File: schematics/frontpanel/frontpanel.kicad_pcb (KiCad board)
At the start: 2 copper layers, 72.4 x 21.6 mm, 10 parts, among them J1 Conn_01x02_Male, J2 Conn_01x02_Male, J3 Conn_01x03_Male, J4 Conn_01x03_Male, SW1 SW_Push, SW2 SW_Push

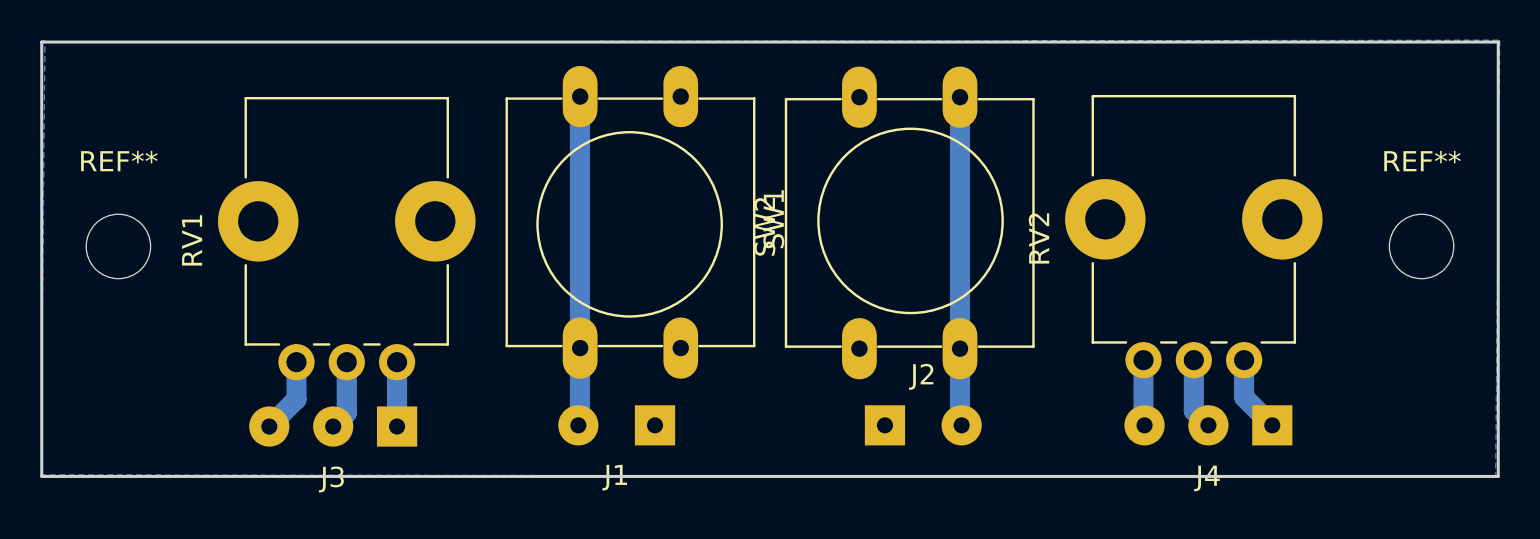
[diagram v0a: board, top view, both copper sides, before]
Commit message: PCBs updated
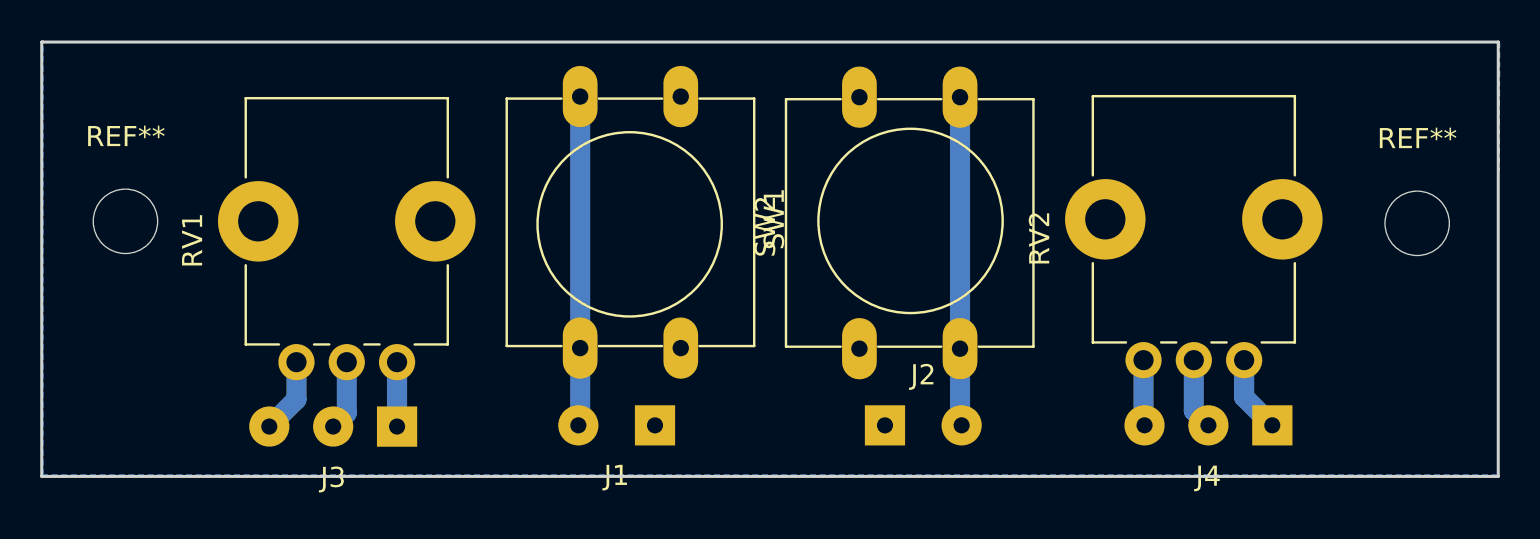
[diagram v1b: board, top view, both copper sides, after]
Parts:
- removed the REF** at (109.2, 120.7)
- removed the REF** at (44.5, 120.7)
- added REF**: MountingHole_3.2mm_M3, MountingHole:MountingHole_3.2mm_M3, F.Cu at (109.0, 119.5)
- added REF**: MountingHole_3.2mm_M3, MountingHole:MountingHole_3.2mm_M3, F.Cu at (44.8, 119.4)
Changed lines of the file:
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@@
     (thickness 1.6)
     (drawings 6)
-    (tracks 18)
+    (tracks 19)
     (zones 0)
     (modules 10)
@@
     (last_trace_width 1)
     (trace_clearance 0.5)
-    (zone_clearance 0.508)
+    (zone_clearance 0.6)
     (zone_45_only no)
     (trace_min 0.2)
@@
     (visible_elements FFFFFF7F)
     (pcbplotparams
-      (layerselection 0x010fc_ffffffff)
+      (layerselection 0x00000_fffffffe)
       (usegerberextensions false)
       (usegerberattributes false)
       (usegerberadvancedattributes false)
       (creategerberjobfile false)
-      (excludeedgelayer true)
+      (excludeedgelayer false)
       (linewidth 0.100000)
       (plotframeref false)
@@
       (hpglpenspeed 20)
       (hpglpendiameter 15.000000)
-      (psnegative false)
+      (psnegative true)
       (psa4output false)
-      (plotreference true)
-      (plotvalue true)
+      (plotreference false)
+      (plotvalue false)
       (plotinvisibletext false)
-      (padsonsilk false)
+      (padsonsilk true)
       (subtractmaskfromsilk false)
-      (outputformat 1)
+      (outputformat 4)
       (mirror false)
-      (drillshape 1)
+      (drillshape 2)
       (scaleselection 1)
       (outputdirectory ""))
@@
   )
   (module MountingHole:MountingHole_3.2mm_M3 (layer F.Cu)
-    (at 109.22 120.65)
+    (at 109 119.5)
     (descr "Mounting Hole 3.2mm, no annular, M3")
     (tags "mounting hole 3.2mm no annular m3")
@@
   )
   (module MountingHole:MountingHole_3.2mm_M3 (layer F.Cu)
-    (at 44.45 120.65)
+    (at 44.8 119.4)
     (descr "Mounting Hole 3.2mm, no annular, M3")
     (tags "mounting hole 3.2mm no annular m3")
@@
     )
     (pad 1 np_thru_hole circle (at 0 0) (size 3.2 3.2) (drill 3.2) (layers *.Cu *.Mask))
+  )
+  (dimension 72.39 (width 0.3) (layer Dwgs.User)
+    (gr_text "72,390 mm" (at 76.835 139.26) (layer Dwgs.User)
+      (effects (font (size 1.5 1.5) (thickness 0.3)))
+    )
+    (feature1 (pts (xy 113.03 132.08) (xy 113.03 137.746421)))
+    (feature2 (pts (xy 40.64 132.08) (xy 40.64 137.746421)))
+    (crossbar (pts (xy 40.64 137.16) (xy 113.03 137.16)))
+    (arrow1a (pts (xy 113.03 137.16) (xy 111.903496 137.746421)))
+    (arrow1b (pts (xy 113.03 137.16) (xy 111.903496 136.573579)))
+    (arrow2a (pts (xy 40.64 137.16) (xy 41.766504 137.746421)))
+    (arrow2b (pts (xy 40.64 137.16) (xy 41.766504 136.573579)))
   )
   (dimension 21.59 (width 0.3) (layer Dwgs.User)
@@
     (arrow2b (pts (xy 35.56 132.08) (xy 34.973579 130.953496)))
   )
-  (dimension 72.39 (width 0.3) (layer Dwgs.User)
-    (gr_text "72,390 mm" (at 76.835 139.26) (layer Dwgs.User)
-      (effects (font (size 1.5 1.5) (thickness 0.3)))
-    )
-    (feature1 (pts (xy 113.03 132.08) (xy 113.03 137.746421)))
-    (feature2 (pts (xy 40.64 132.08) (xy 40.64 137.746421)))
-    (crossbar (pts (xy 40.64 137.16) (xy 113.03 137.16)))
-    (arrow1a (pts (xy 113.03 137.16) (xy 111.903496 137.746421)))
-    (arrow1b (pts (xy 113.03 137.16) (xy 111.903496 136.573579)))
-    (arrow2a (pts (xy 40.64 137.16) (xy 41.766504 137.746421)))
-    (arrow2b (pts (xy 40.64 137.16) (xy 41.766504 136.573579)))
-  )
   (gr_line (start 40.64 132.08) (end 40.64 110.49) (layer Edge.Cuts) (width 0.15))
   (gr_line (start 113.03 132.08) (end 40.64 132.08) (layer Edge.Cuts) (width 0.15))
@@
   (segment (start 81.08 113.03) (end 81.28 113.23) (width 1) (layer B.Cu) (net 1))
   (segment (start 67.39 129.46) (end 67.31 129.54) (width 1) (layer B.Cu) (net 2))
-  (segment (start 67.39 113.03) (end 67.39 129.46) (width 1) (layer B.Cu) (net 2))
+  (segment (start 67.4 129.45) (end 67.31 129.54) (width 1) (layer B.Cu) (net 2))
+  (segment (start 67.4 113.2) (end 67.4 129.45) (width 1) (layer B.Cu) (net 2))
   (segment (start 58.3 126.4) (end 58.3 129.6) (width 1) (layer B.Cu) (net 3))
   (segment (start 55.8 128.925) (end 55.125 129.6) (width 1) (layer B.Cu) (net 4))
@@
   (segment (start 86.28 113.23) (end 86.28 129.46) (width 1) (layer B.Cu) (net 9))
   (zone (net 1) (net_name "Net-(J1-Pad1)") (layer B.Cu) (hatch edge 0.508)
-    (connect_pads (clearance 0.508))
+    (connect_pads (clearance 0.6))
     (min_thickness 0.254)
     (fill yes (arc_segments 16) (thermal_gap 0.508) (thermal_bridge_width 0.508))
     (polygon
       (pts
-        (xy 40.7 110.5) (xy 113.1 110.4) (xy 112.9 132.1) (xy 40.6 132) (xy 40.8 110.4)
-        (xy 40.6 110.5) (xy 40.8 110.5)
+        (xy 40.775 110.5) (xy 113.1 110.5) (xy 113 132) (xy 40.7 132) (xy 40.7 110.4)
       )
     )
